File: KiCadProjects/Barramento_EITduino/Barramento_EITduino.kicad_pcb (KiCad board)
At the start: 2 copper layers, 90 x 100 mm, 3 parts, among them J2 tensoes, J3 sinais analogicos, J4 comunicacao / sinais digitais

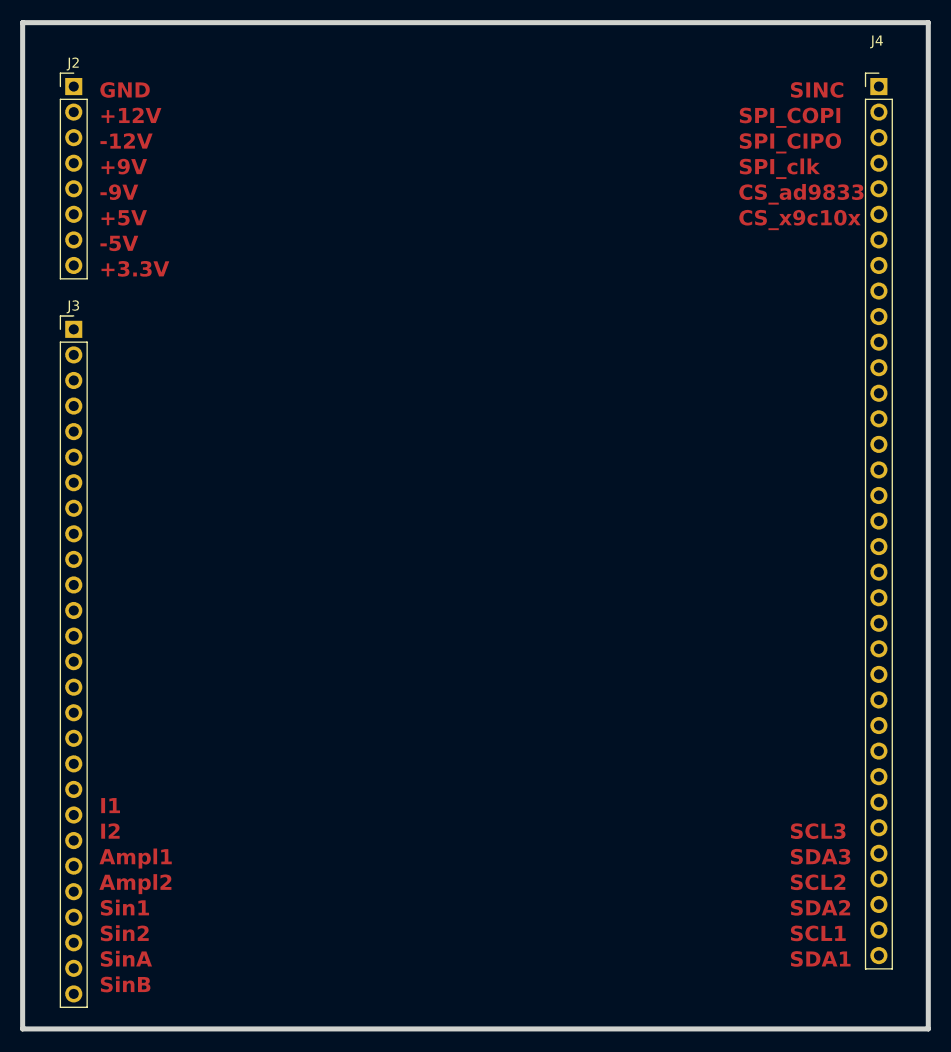
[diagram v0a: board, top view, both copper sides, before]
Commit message: Descrição do barramento: esquemático
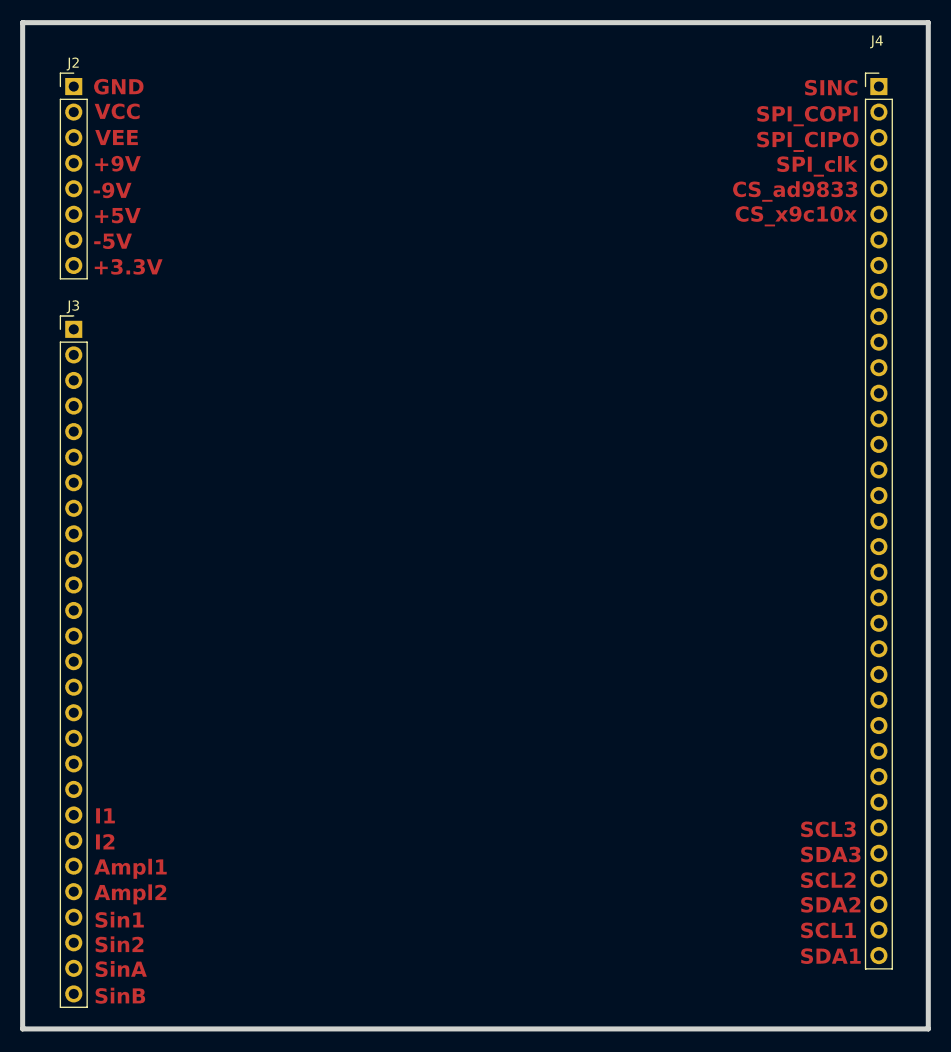
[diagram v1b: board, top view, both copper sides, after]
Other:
- board text added: "VCC"
- board text added: "VEE"
- board text removed: "+12V"
- board text removed: "-12V"
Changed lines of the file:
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@@
   (gr_line (start 101.6 50.8) (end 101.6 150.7998)
     (stroke (width 0.5) (type default)) (layer "Edge.Cuts"))
-  (gr_text "SDA1" (at 177.8 144.78) (layer "F.Cu")
+  (gr_text "SDA1" (at 178.816 144.5) (layer "F.Cu")
     (effects (font (size 1.5 1.5) (thickness 0.3) bold) (justify left bottom))
   )
-  (gr_text "SinA" (at 109.22 144.78) (layer "F.Cu")
+  (gr_text "SinA" (at 108.712 145.796) (layer "F.Cu")
     (effects (font (size 1.5 1.5) (thickness 0.3) bold) (justify left bottom))
   )
-  (gr_text "SPI_CIPO\n" (at 172.72 63.5) (layer "F.Cu")
+  (gr_text "SPI_CIPO\n" (at 174.45 63.35) (layer "F.Cu")
     (effects (font (size 1.5 1.5) (thickness 0.3) bold) (justify left bottom))
   )
-  (gr_text "CS_x9c10x\n" (at 172.72 71.12) (layer "F.Cu")
+  (gr_text "CS_x9c10x\n" (at 172.35 70.75) (layer "F.Cu")
     (effects (font (size 1.5 1.5) (thickness 0.3) bold) (justify left bottom))
   )
-  (gr_text "-9V" (at 109.22 68.58) (layer "F.Cu")
+  (gr_text "-9V" (at 108.55 68.4) (layer "F.Cu")
     (effects (font (size 1.5 1.5) (thickness 0.3) bold) (justify left bottom))
   )
-  (gr_text "CS_ad9833" (at 172.72 68.58) (layer "F.Cu")
+  (gr_text "CS_ad9833" (at 172.1 68.3) (layer "F.Cu")
     (effects (font (size 1.5 1.5) (thickness 0.3) bold) (justify left bottom))
   )
-  (gr_text "+3.3V" (at 109.22 76.2) (layer "F.Cu")
+  (gr_text "+3.3V" (at 108.55 76) (layer "F.Cu")
     (effects (font (size 1.5 1.5) (thickness 0.3) bold) (justify left bottom))
   )
-  (gr_text "Sin1" (at 109.22 139.7) (layer "F.Cu")
+  (gr_text "Sin1" (at 108.7 140.9) (layer "F.Cu")
     (effects (font (size 1.5 1.5) (thickness 0.3) bold) (justify left bottom))
   )
-  (gr_text "+5V\n" (at 109.22 71.12) (layer "F.Cu")
+  (gr_text "+5V\n" (at 108.6 70.9) (layer "F.Cu")
     (effects (font (size 1.5 1.5) (thickness 0.3) bold) (justify left bottom))
   )
-  (gr_text "SCL2" (at 177.8 137.16) (layer "F.Cu")
+  (gr_text "SCL2" (at 178.816 136.95) (layer "F.Cu")
     (effects (font (size 1.5 1.5) (thickness 0.3) bold) (justify left bottom))
   )
-  (gr_text "-5V" (at 109.22 73.66) (layer "F.Cu")
+  (gr_text "-5V" (at 108.6 73.45) (layer "F.Cu")
     (effects (font (size 1.5 1.5) (thickness 0.3) bold) (justify left bottom))
   )
-  (gr_text "GND" (at 109.22 58.42) (layer "F.Cu")
+  (gr_text "GND" (at 108.6 58.1) (layer "F.Cu")
     (effects (font (size 1.5 1.5) (thickness 0.3) bold) (justify left bottom))
   )
-  (gr_text "SDA3" (at 177.8 134.62) (layer "F.Cu")
+  (gr_text "SDA3" (at 178.816 134.4) (layer "F.Cu")
     (effects (font (size 1.5 1.5) (thickness 0.3) bold) (justify left bottom))
   )
-  (gr_text "Ampl2" (at 109.22 137.16) (layer "F.Cu")
+  (gr_text "Ampl2" (at 108.712 138.176) (layer "F.Cu")
     (effects (font (size 1.5 1.5) (thickness 0.3) bold) (justify left bottom))
   )
-  (gr_text "SINC" (at 177.8 58.42) (layer "F.Cu")
+  (gr_text "SINC" (at 179.2 58.2) (layer "F.Cu")
     (effects (font (size 1.5 1.5) (thickness 0.3) bold) (justify left bottom))
   )
-  (gr_text "+12V\n" (at 109.22 60.96) (layer "F.Cu")
+  (gr_text "VCC" (at 108.75 60.55) (layer "F.Cu")
     (effects (font (size 1.5 1.5) (thickness 0.3) bold) (justify left bottom))
   )
-  (gr_text "-12V\n" (at 109.22 63.5) (layer "F.Cu")
+  (gr_text "VEE\n" (at 108.8 63.15) (layer "F.Cu")
     (effects (font (size 1.5 1.5) (thickness 0.3) bold) (justify left bottom))
   )
-  (gr_text "I2\n" (at 109.22 132.08) (layer "F.Cu")
+  (gr_text "I2\n" (at 108.7 133.15) (layer "F.Cu")
     (effects (font (size 1.5 1.5) (thickness 0.3) bold) (justify left bottom))
   )
-  (gr_text "SinB" (at 109.22 147.32) (layer "F.Cu")
+  (gr_text "SinB" (at 108.7 148.45) (layer "F.Cu")
     (effects (font (size 1.5 1.5) (thickness 0.3) bold) (justify left bottom))
   )
-  (gr_text "SDA2" (at 177.8 139.7) (layer "F.Cu")
+  (gr_text "SDA2" (at 178.816 139.4) (layer "F.Cu")
     (effects (font (size 1.5 1.5) (thickness 0.3) bold) (justify left bottom))
   )
-  (gr_text "SPI_clk\n" (at 172.72 66.04) (layer "F.Cu")
+  (gr_text "SPI_clk\n" (at 176.45 65.8) (layer "F.Cu")
     (effects (font (size 1.5 1.5) (thickness 0.3) bold) (justify left bottom))
   )
-  (gr_text "I1" (at 109.22 129.54) (layer "F.Cu")
+  (gr_text "I1" (at 108.712 130.556) (layer "F.Cu")
     (effects (font (size 1.5 1.5) (thickness 0.3) bold) (justify left bottom))
   )
-  (gr_text "Sin2\n" (at 109.22 142.24) (layer "F.Cu")
+  (gr_text "Sin2\n" (at 108.7 143.35) (layer "F.Cu")
     (effects (font (size 1.5 1.5) (thickness 0.3) bold) (justify left bottom))
   )
-  (gr_text "+9V\n" (at 109.22 66.04) (layer "F.Cu")
+  (gr_text "+9V\n" (at 108.6 65.75) (layer "F.Cu")
     (effects (font (size 1.5 1.5) (thickness 0.3) bold) (justify left bottom))
   )
-  (gr_text "SCL1\n" (at 177.8 142.24) (layer "F.Cu")
+  (gr_text "SCL1\n" (at 178.816 141.94) (layer "F.Cu")
     (effects (font (size 1.5 1.5) (thickness 0.3) bold) (justify left bottom))
   )
-  (gr_text "SPI_COPI\n" (at 172.72 60.96) (layer "F.Cu")
+  (gr_text "SPI_COPI\n" (at 174.45 60.8) (layer "F.Cu")
     (effects (font (size 1.5 1.5) (thickness 0.3) bold) (justify left bottom))
   )
-  (gr_text "SCL3" (at 177.8 132.08) (layer "F.Cu")
+  (gr_text "SCL3" (at 178.816 131.9) (layer "F.Cu")
     (effects (font (size 1.5 1.5) (thickness 0.3) bold) (justify left bottom))
   )
-  (gr_text "Ampl1" (at 109.22 134.62) (layer "F.Cu")
+  (gr_text "Ampl1" (at 108.712 135.636) (layer "F.Cu")
     (effects (font (size 1.5 1.5) (thickness 0.3) bold) (justify left bottom))
   )
